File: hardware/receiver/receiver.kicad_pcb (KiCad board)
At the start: 4 copper layers, 20 x 44 mm, 18 parts, among them J1 USB-C HRO TYPE-C-31-M-12, J2 SWD: VDD / SWDIO / SWDCLK / G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, SW1 PAIR TL3342, SW2 RESET TL3342, U1 MDBT50Q-1MV2, U2 USBLC6-2SC6, U3 TLV70030DDCR, Y1 32.768kHz 12.5pF ABS07

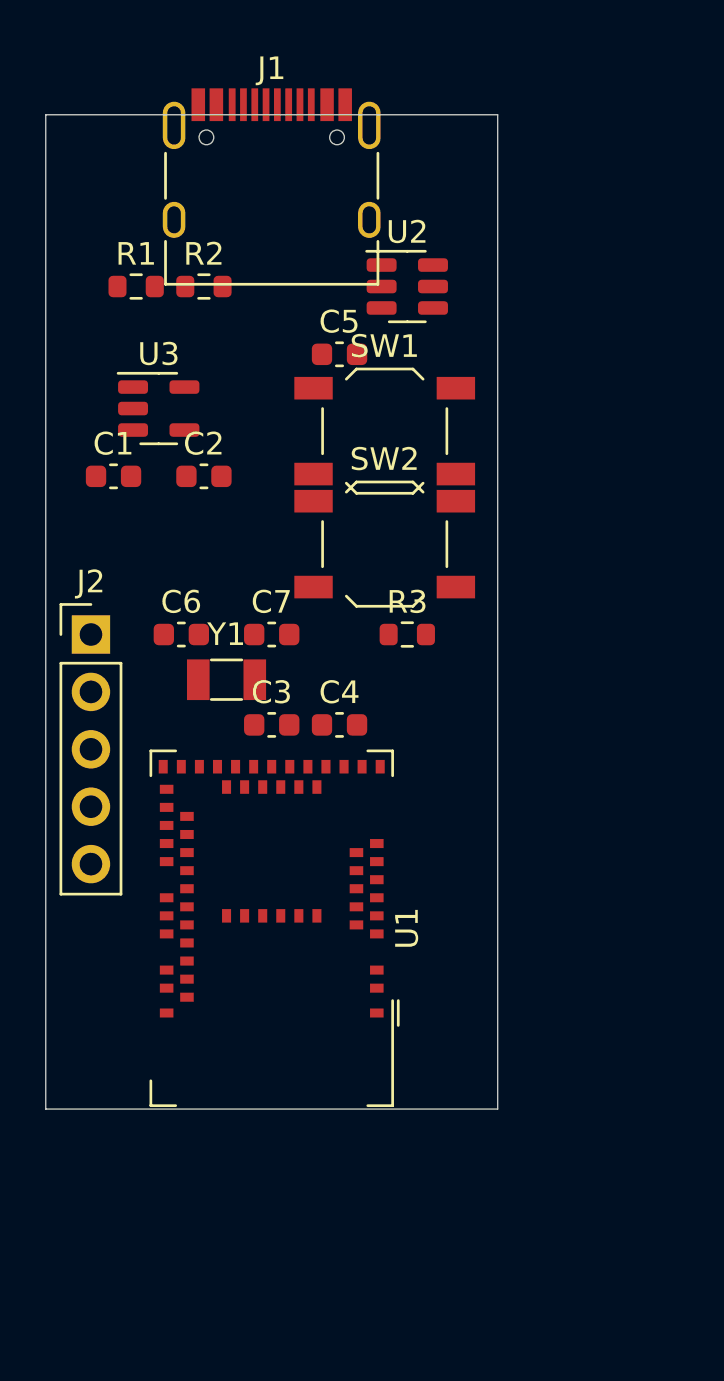
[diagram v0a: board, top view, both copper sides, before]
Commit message: Route A1 prototype boards and build native firmware; bench validation pending
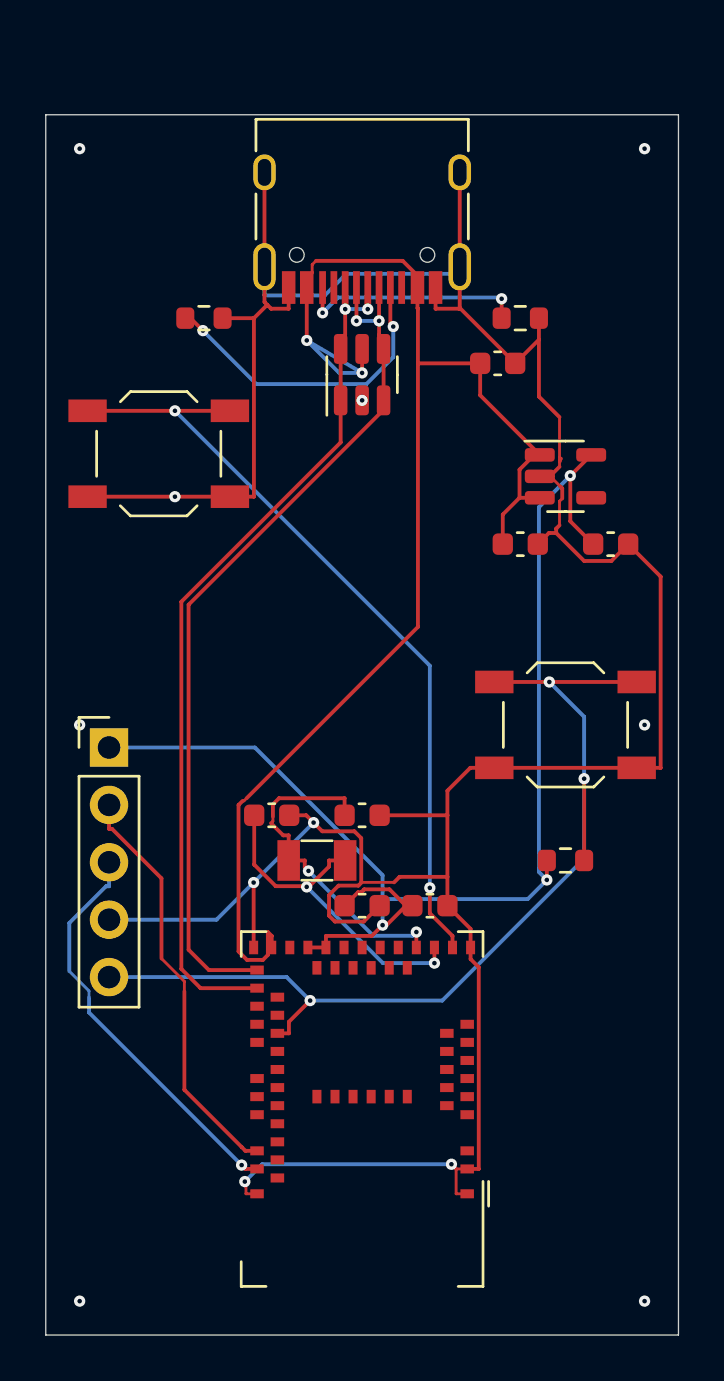
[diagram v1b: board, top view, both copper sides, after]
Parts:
- moved C1 18.2 mm to (21.0, 19.0)
- moved C2 18.2 mm to (25.0, 19.0)
- moved U3 18.2 mm to (23.0, 16.0)
- moved R2 14.1 mm to (21.0, 9.00)
- moved R3 12.2 mm to (23.0, 33.0)
- moved SW2 11.3 mm to (23.0, 27.0)
- moved SW1 10.0 mm to (5.00, 15.0)
- moved C3 8.94 mm to (14.0, 35.0)
- moved C4 8.94 mm to (17.0, 35.0)
- moved C6 8.94 mm to (10.0, 31.0)
- moved C7 8.94 mm to (14.0, 31.0)
- moved U1 8.94 mm to (14.0, 44.0)
- moved Y1 8.94 mm to (12.0, 33.0)
- moved C5 7.01 mm to (20.0, 11.0)
- moved J2 5.06 mm to (2.80, 28.0)
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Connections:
- net CC1 renamed /CC1
- net CC2 renamed /CC2
- net GND renamed /GND
- net LF_XL1 renamed /LF_XL1
- net LF_XL2 renamed /LF_XL2
- net MCU_RESET renamed /MCU_RESET
- net PAIR renamed /PAIR
- net SWDCLK renamed /SWDCLK
- net SWDIO renamed /SWDIO
- net USB_DM renamed /USB_DM
- net USB_DP renamed /USB_DP
- net USB_VBUS renamed /USB_VBUS
- net VDD_3V0 renamed /VDD_3V0
- J1 pad A8: (no net) -> unconnected-(J1-PadA8)
- J1 pad B8: (no net) -> unconnected-(J1-PadB8)
- U1 pad 10: (no net) -> unconnected-(U1-P0.29/AIN5-Pad10)
- U1 pad 11: (no net) -> unconnected-(U1-P0.02/AIN0-Pad11)
- U1 pad 12: (no net) -> unconnected-(U1-P0.31/AIN7-Pad12)
- U1 pad 13: (no net) -> unconnected-(U1-P0.28/AIN4-Pad13)
- U1 pad 14: (no net) -> unconnected-(U1-P0.30/AIN6-Pad14)
- U1 pad 19: (no net) -> unconnected-(U1-P0.26-Pad19)
- U1 pad 20: (no net) -> unconnected-(U1-P0.04/AIN2-Pad20)
- U1 pad 21: (no net) -> unconnected-(U1-P0.05/AIN3-Pad21)
- U1 pad 22: (no net) -> unconnected-(U1-P0.06-Pad22)
- U1 pad 23: (no net) -> unconnected-(U1-TRACECLK/P0.07-Pad23)
- U1 pad 24: (no net) -> unconnected-(U1-P0.08-Pad24)
- U1 pad 25: (no net) -> unconnected-(U1-P1.08-Pad25)
- U1 pad 26: (no net) -> unconnected-(U1-TRACEDATA3/P1.09-Pad26)
- U1 pad 27: (no net) -> unconnected-(U1-TRACEDATA2/P0.11-Pad27)
- U1 pad 29: (no net) -> unconnected-(U1-TRACEDATA1/P0.12-Pad29)
- U1 pad 3: (no net) -> unconnected-(U1-P1.10-Pad3)
- U1 pad 31: (no net) -> unconnected-(U1-DCCH-Pad31)
- U1 pad 36: (no net) -> unconnected-(U1-P0.14-Pad36)
- U1 pad 37: (no net) -> unconnected-(U1-P0.13-Pad37)
- U1 pad 38: (no net) -> unconnected-(U1-P0.16-Pad38)
- U1 pad 39: (no net) -> unconnected-(U1-P0.15-Pad39)
- U1 pad 4: (no net) -> unconnected-(U1-P1.11-Pad4)
- U1 pad 41: (no net) -> unconnected-(U1-P0.17-Pad41)
- U1 pad 42: (no net) -> unconnected-(U1-P0.19-Pad42)
- U1 pad 43: (no net) -> unconnected-(U1-P0.21-Pad43)
- U1 pad 44: (no net) -> unconnected-(U1-P0.20-Pad44)
- U1 pad 45: (no net) -> unconnected-(U1-P0.23-Pad45)
- U1 pad 46: (no net) -> unconnected-(U1-P0.22-Pad46)
- U1 pad 47: (no net) -> unconnected-(U1-TRACEDATA0/P1.00-Pad47)
- U1 pad 48: (no net) -> unconnected-(U1-P0.24-Pad48)
- U1 pad 49: (no net) -> unconnected-(U1-P0.25-Pad49)
- U1 pad 5: (no net) -> unconnected-(U1-P1.12-Pad5)
- U1 pad 50: (no net) -> unconnected-(U1-P1.02-Pad50)
- U1 pad 52: (no net) -> unconnected-(U1-P0.09/NFC1-Pad52)
- U1 pad 54: (no net) -> unconnected-(U1-P0.10/NFC2-Pad54)
- U1 pad 56: (no net) -> unconnected-(U1-P1.04-Pad56)
- U1 pad 57: (no net) -> unconnected-(U1-P1.06-Pad57)
- U1 pad 58: (no net) -> unconnected-(U1-P1.07-Pad58)
- U1 pad 59: (no net) -> unconnected-(U1-P1.05-Pad59)
- U1 pad 6: (no net) -> unconnected-(U1-P1.13-Pad6)
- U1 pad 60: (no net) -> unconnected-(U1-P1.03-Pad60)
- U1 pad 61: (no net) -> unconnected-(U1-P1.01-Pad61)
- U1 pad 7: (no net) -> unconnected-(U1-P1.14-Pad7)
- U1 pad 8: (no net) -> unconnected-(U1-P1.15-Pad8)
- U1 pad 9: (no net) -> unconnected-(U1-P0.03/AIN1-Pad9)
- U3 pad 4: (no net) -> unconnected-(U3-Pad4)
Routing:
- net /GND: track 0.00 -> 147.2 mm, vias 0 -> 12
- net /USB_VBUS: track 0.00 -> 65.4 mm, vias 0 -> 2
- net /VDD_3V0: track 0.00 -> 57.5 mm, vias 0 -> 3
- net /MCU_RESET: track 0.00 -> 44.8 mm, vias 0 -> 3
- net /USB_DM: track 0.00 -> 38.8 mm, vias 0 -> 2
- net /USB_DP: track 0.00 -> 38.8 mm, vias 0 -> 2
- net /PAIR: track 0.00 -> 35.1 mm, vias 0 -> 2
- net /SWDIO: track 0.00 -> 18.4 mm
- net /SWDCLK: track 0.00 -> 18.1 mm, vias 0 -> 1
- net /LF_XL1: track 0.00 -> 15.0 mm, vias 0 -> 2
- net /LF_XL2: track 0.00 -> 15.0 mm, vias 0 -> 2
- net /CC1: track 0.00 -> 14.0 mm, vias 0 -> 2
- net /CC2: track 0.00 -> 10.2 mm, vias 0 -> 2
- added copper zone on In1.Cu, net /GND
- added copper zone on In2.Cu, net /GND
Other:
- board size 20 x 44 mm -> 28 x 54 mm
- board text added: "A1 ROUTED PROTOTYPE - PHYSICAL TESTS NOT RUN"
- board text added: "OPENMICE RECEIVER A1"
- board text removed: "OPENMICE RECEIVER A0"
- board text removed: "PLACEMENT DRAFT - NOT FOR FABRICATION"
